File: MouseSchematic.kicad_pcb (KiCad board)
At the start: 2 copper layers, 83.2 x 82.7 mm, 69 parts, among them IC1 AZ1117IH-3.3TRG1, J1 Right Header, J2 Left Header, J4 JST1, J5 JST2, J6 Programming Header, Q1 IR Receiver, Q2 IR Receiver, Q3 IR Receiver, Q4 IR Receiver, Q5 MOSFET, Q6 MOSFET, Q7 MOSFET, Q8 MOSFET, SW1 Button, U1 STM32F205RGTx, U2 L293DD

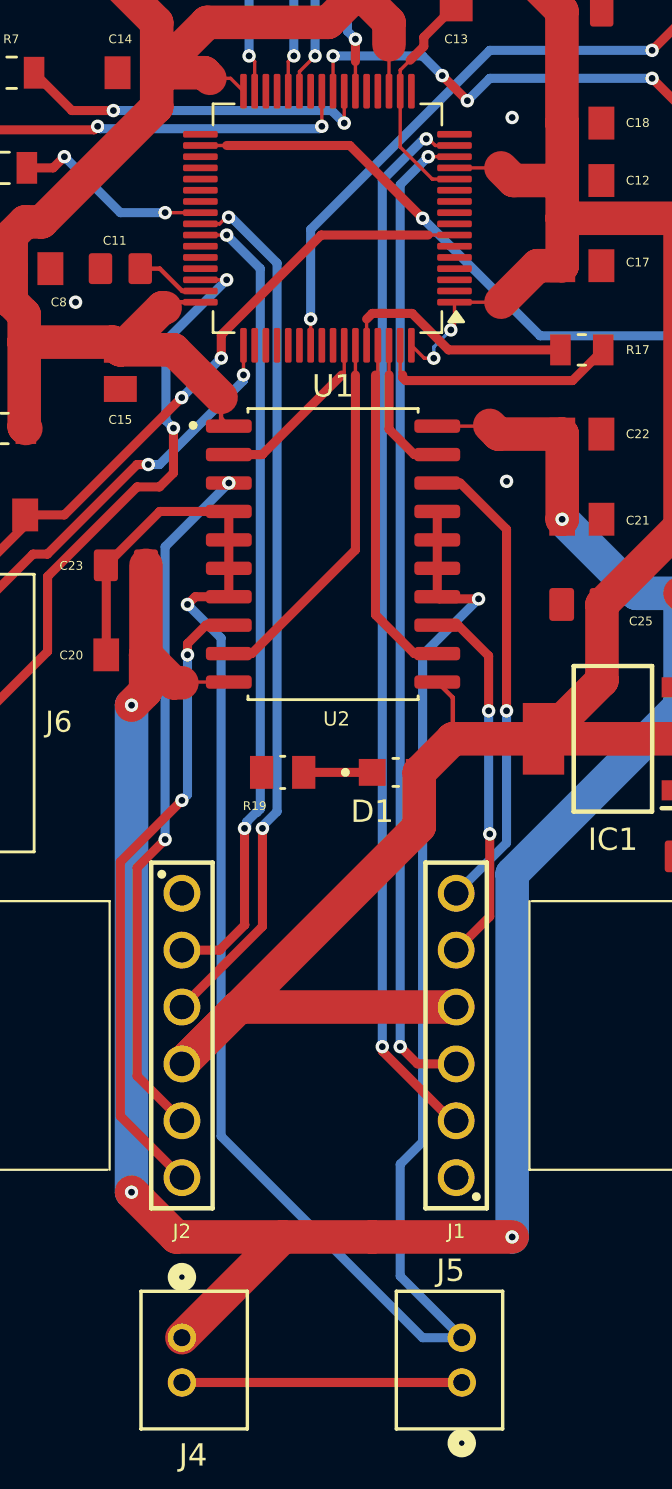
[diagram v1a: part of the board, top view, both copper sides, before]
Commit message: Final PCB
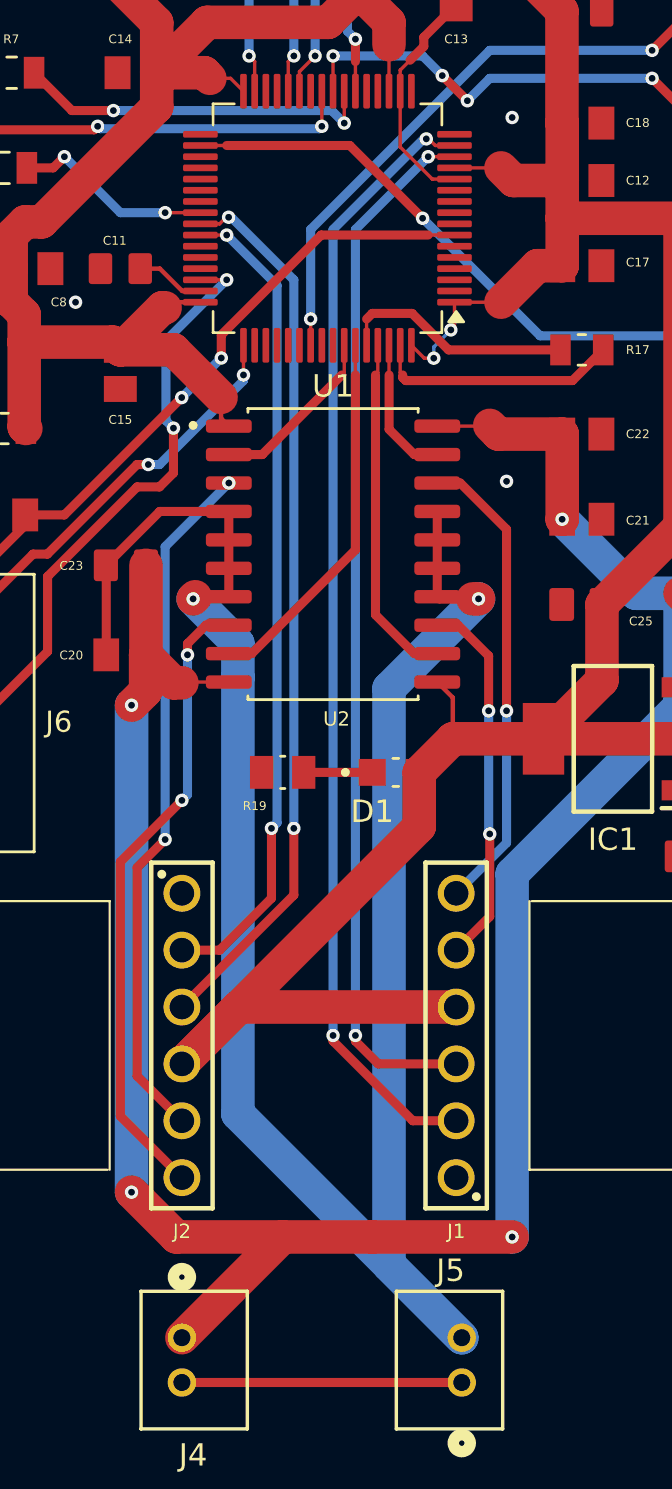
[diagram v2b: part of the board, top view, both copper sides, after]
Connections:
- J5 pad 2: MGND -> GND
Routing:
- net PA1: track 47.6 -> 50.4 mm
- net PA0: track 44.3 -> 46.9 mm
- net MGND: track 96.4 -> 95.6 mm
- net PA9: track 36.2 -> 36.8 mm
- net PA8: track 39.4 -> 40.0 mm
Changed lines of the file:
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@@
 			(layers "*.Cu" "*.Mask")
 			(remove_unused_layers no)
-			(net 81 "MGND")
+			(net 1 "GND")
 			(pinfunction "2")
 			(pintype "unspecified")
@@
 	)
 	(segment
-		(start 164.75 129.27)
-		(end 163.02 129.27)
+		(start 161.27 129.27)
+		(end 164.75 129.27)
 		(width 0.4064)
 		(layer "F.Cu")
@@
 	)
 	(segment
-		(start 163.02 129.27)
-		(end 162.25 128.5)
+		(start 160.25 128.25)
+		(end 161.27 129.27)
+		(width 0.4064)
+		(layer "F.Cu")
+		(net 9)
+	)
+	(segment
+		(start 160.25 128)
+		(end 160.25 128.25)
 		(width 0.4064)
 		(layer "F.Cu")
@@
 	)
 	(via
-		(at 162.25 128.5)
+		(at 160.25 128)
 		(size 0.6)
 		(drill 0.3)
@@
 	)
 	(segment
-		(start 162.25 128.5)
-		(end 162.25 90)
+		(start 160.25 92)
+		(end 163.5 88.75)
 		(width 0.4064)
 		(layer "B.Cu")
@@
 	)
 	(segment
-		(start 162.25 90)
-		(end 163.5 88.75)
+		(start 160.25 128)
+		(end 160.25 92)
 		(width 0.4064)
 		(layer "B.Cu")
@@
 	)
 	(segment
-		(start 164.56411 131.81)
-		(end 161.449997 128.695887)
-		(width 0.4064)
-		(layer "F.Cu")
-		(net 10)
-	)
-	(segment
-		(start 161.449997 128.695887)
-		(end 161.449997 128.5)
+		(start 159.25 128.25)
+		(end 162.81 131.81)
 		(width 0.4064)
 		(layer "F.Cu")
@@
 	)
 	(segment
-		(start 164.75 131.81)
-		(end 164.56411 131.81)
+		(start 162.81 131.81)
+		(end 164.75 131.81)
+		(width 0.4064)
+		(layer "F.Cu")
+		(net 10)
+	)
+	(segment
+		(start 159.25 128)
+		(end 159.25 128.25)
 		(width 0.4064)
 		(layer "F.Cu")
@@
 	)
 	(via
-		(at 161.449997 128.5)
+		(at 159.25 128)
 		(size 0.6)
 		(drill 0.3)
@@
 	)
 	(segment
-		(start 161.449997 128.5)
-		(end 161.449997 89.805527)
+		(start 159.25 128)
+		(end 159.25 92.005524)
 		(width 0.4064)
 		(layer "B.Cu")
@@
 	)
 	(segment
-		(start 161.449997 89.805527)
+		(start 159.25 92.005524)
 		(end 163.300947 87.954577)
 		(width 0.4064)
@@
 	)
 	(segment
-		(start 156.096803 123.133197)
-		(end 156.096803 118.75)
+		(start 157.5 121.73)
+		(end 152.5 126.73)
 		(width 0.4064)
 		(layer "F.Cu")
@@
 	)
 	(segment
-		(start 152.5 126.73)
-		(end 156.096803 123.133197)
+		(start 157.5 118.75)
+		(end 157.5 121.73)
 		(width 0.4064)
 		(layer "F.Cu")
@@
 	)
 	(via
-		(at 156.096803 118.75)
+		(at 157.5 118.75)
 		(size 0.6)
 		(drill 0.3)
@@
 	)
 	(segment
-		(start 156.75 118)
-		(end 156.75 93.50411)
-		(width 0.4064)
-		(layer "B.Cu")
-		(net 14)
-	)
-	(segment
-		(start 156 118.75)
-		(end 156.75 118)
+		(start 157.5 94.25411)
+		(end 154.700469 91.454579)
 		(width 0.4064)
 		(layer "B.Cu")
@@
 	)
 	(segment
-		(start 156.75 93.50411)
-		(end 154.700469 91.454579)
+		(start 157.5 118.75)
+		(end 157.5 94.25411)
 		(width 0.4064)
 		(layer "B.Cu")
@@
 	(segment
 		(start 154.181006 124.19)
-		(end 155.310503 123.060503)
+		(end 152.5 124.19)
 		(width 0.4064)
 		(layer "F.Cu")
@@
 	)
 	(segment
-		(start 155.310503 123.060503)
-		(end 155.2968 123.0468)
+		(start 156.5 121.871006)
+		(end 154.181006 124.19)
 		(width 0.4064)
 		(layer "F.Cu")
@@
 	)
 	(segment
-		(start 152.5 124.19)
-		(end 154.181006 124.19)
+		(start 156.5 118.75)
+		(end 156.5 121.871006)
 		(width 0.4064)
 		(layer "F.Cu")
@@
 		(net 15)
 	)
-	(segment
-		(start 155.2968 123.0468)
-		(end 155.2968 118.75)
-		(width 0.4064)
-		(layer "F.Cu")
-		(net 15)
-	)
 	(via
-		(at 155.2968 118.75)
+		(at 156.5 118.75)
 		(size 0.6)
 		(drill 0.3)
@@
 	)
 	(segment
-		(start 155.845206 118.0458)
-		(end 156 117.891006)
+		(start 156.75 118.5)
+		(end 156.75 94.5)
 		(width 0.4064)
 		(layer "B.Cu")
@@
 	)
 	(segment
-		(start 156 93.75)
+		(start 156.75 94.5)
 		(end 154.5 92.25)
 		(width 0.4064)
@@
 	)
 	(segment
-		(start 155.2992 118.75)
-		(end 155.3926 118.6566)
-		(width 0.4064)
-		(layer "B.Cu")
-		(net 15)
-	)
-	(segment
-		(start 155.805113 118.0458)
-		(end 155.845206 118.0458)
-		(width 0.4064)
-		(layer "B.Cu")
-		(net 15)
-	)
-	(segment
-		(start 155.3926 118.6566)
-		(end 155.3926 118.498406)
-		(width 0.4064)
-		(layer "B.Cu")
-		(net 15)
-	)
-	(segment
-		(start 155.392603 118.498403)
-		(end 155.392603 118.45831)
-		(width 0.4064)
-		(layer "B.Cu")
-		(net 15)
-	)
-	(segment
-		(start 155.3926 118.498406)
-		(end 155.392603 118.498403)
-		(width 0.4064)
-		(layer "B.Cu")
-		(net 15)
-	)
-	(segment
-		(start 156 117.891006)
-		(end 156 93.75)
-		(width 0.4064)
-		(layer "B.Cu")
-		(net 15)
-	)
-	(segment
-		(start 155.392603 118.45831)
-		(end 155.805113 118.0458)
+		(start 156.5 118.75)
+		(end 156.75 118.5)
 		(width 0.4064)
 		(layer "B.Cu")
@@
 	)
 	(segment
-		(start 153.095 108.405)
-		(end 152.75 108.75)
-		(width 0.4064)
-		(layer "F.Cu")
-		(net 81)
-	)
-	(segment
 		(start 154.595 108.405)
 		(end 153.095 108.405)
@@
 	(segment
 		(start 163.905 108.405)
-		(end 164 108.5)
+		(end 163.905 104.595)
 		(width 0.4064)
 		(layer "F.Cu")
@@
 	)
 	(segment
-		(start 164 108.5)
-		(end 165.75 108.5)
+		(start 149.105 107)
+		(end 151.51 104.595)
 		(width 0.4064)
 		(layer "F.Cu")
@@
 	)
 	(segment
-		(start 163.905 108.405)
-		(end 163.905 104.595)
+		(start 149.12 107.015)
+		(end 149.105 107)
 		(width 0.4064)
 		(layer "F.Cu")
@@
 	)
 	(segment
-		(start 149.105 107)
-		(end 151.51 104.595)
+		(start 164 108.5)
+		(end 165.5 108.5)
 		(width 0.4064)
 		(layer "F.Cu")
@@
 	)
 	(segment
-		(start 149.12 107.015)
-		(end 149.105 107)
+		(start 154.595 104.595)
+		(end 154.595 105.865)
 		(width 0.4064)
 		(layer "F.Cu")
@@
 	)
 	(segment
-		(start 154.595 104.595)
-		(end 154.595 105.865)
-		(width 0.4064)
+		(start 153 108.5)
+		(end 153.095 108.405)
+		(width 1.5)
 		(layer "F.Cu")
 		(net 81)
@@
 	)
 	(segment
+		(start 163.905 108.405)
+		(end 164 108.5)
+		(width 0.4064)
+		(layer "F.Cu")
+		(net 81)
+	)
+	(segment
+		(start 165.75 108.5)
+		(end 165.5 108.5)
+		(width 1.5)
+		(layer "F.Cu")
+		(net 81)
+	)
+	(segment
 		(start 154.595 105.865)
 		(end 154.595 107.135)
@@
 	)
 	(via
-		(at 152.75 108.75)
+		(at 165.75 108.5)
 		(size 0.6)
 		(drill 0.3)
@@
 	)
 	(via
-		(at 165.75 108.5)
+		(at 153 108.5)
 		(size 0.6)
 		(drill 0.3)
@@
 	)
 	(segment
-		(start 165.75 108.5)
-		(end 163.25 111)
-		(width 0.4064)
-		(layer "B.Cu")
-		(net 81)
-	)
-	(segment
-		(start 163.249999 141.499999)
-		(end 165 141.499999)
-		(width 0.4064)
-		(layer "B.Cu")
-		(net 81)
-	)
-	(segment
-		(start 162.25 133.75)
-		(end 162.25 138.749999)
-		(width 0.4064)
+		(start 165 141.499999)
+		(end 161.75 138.249999)
+		(width 1.5)
 		(layer "B.Cu")
 		(net 81)
 	)
 	(segment
-		(start 163.25 111)
-		(end 163.25 132.75)
-		(width 0.4064)
+		(start 161.75 138.249999)
+		(end 161.75 112.5)
+		(width 1.5)
 		(layer "B.Cu")
 		(net 81)
 	)
 	(segment
-		(start 163.25 132.75)
-		(end 162.25 133.75)
-		(width 0.4064)
+		(start 155 110.5)
+		(end 153 108.5)
+		(width 1.5)
 		(layer "B.Cu")
 		(net 81)
 	)
 	(segment
-		(start 154.25 132.5)
-		(end 163.249999 141.499999)
-		(width 0.4064)
+		(start 165 141.499999)
+		(end 155 131.499999)
+		(width 1.5)
 		(layer "B.Cu")
 		(net 81)
 	)
 	(segment
-		(start 152.75 108.75)
-		(end 154.25 110.25)
-		(width 0.4064)
+		(start 161.75 112.5)
+		(end 165.75 108.5)
+		(width 1.5)
 		(layer "B.Cu")
 		(net 81)
 	)
 	(segment
-		(start 162.25 138.749999)
-		(end 165 141.499999)
-		(width 0.4064)
+		(start 155 112)
+		(end 155 110.5)
+		(width 1.5)
 		(layer "B.Cu")
 		(net 81)
 	)
 	(segment
-		(start 154.25 110.25)
-		(end 154.25 132.5)
-		(width 0.4064)
+		(start 155 131.499999)
+		(end 155 112)
+		(width 1.5)
 		(layer "B.Cu")
 		(net 81)
